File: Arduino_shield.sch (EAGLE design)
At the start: 21 parts

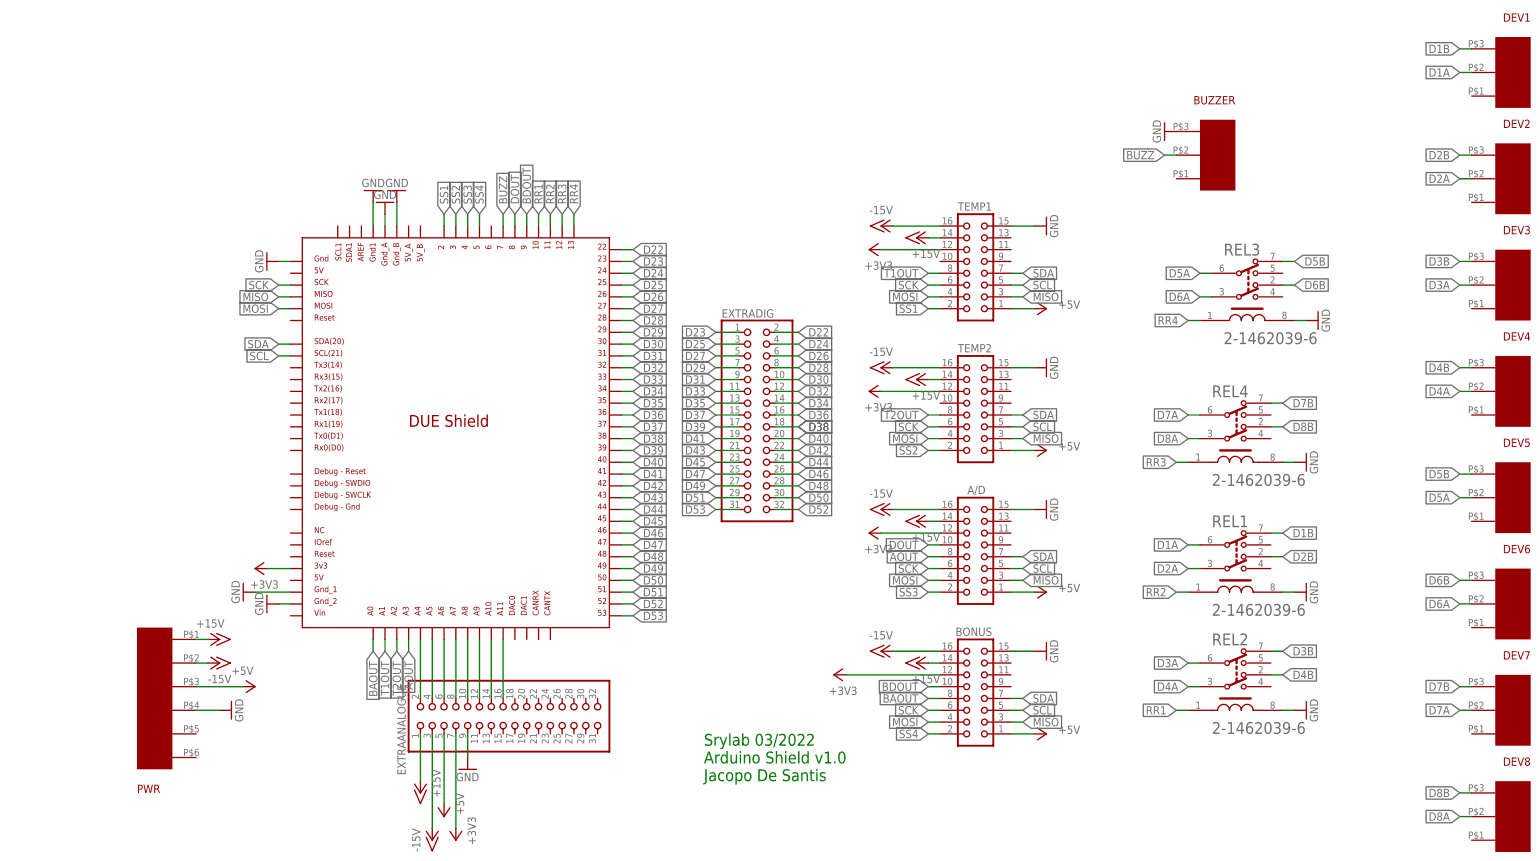
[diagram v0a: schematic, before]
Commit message: production
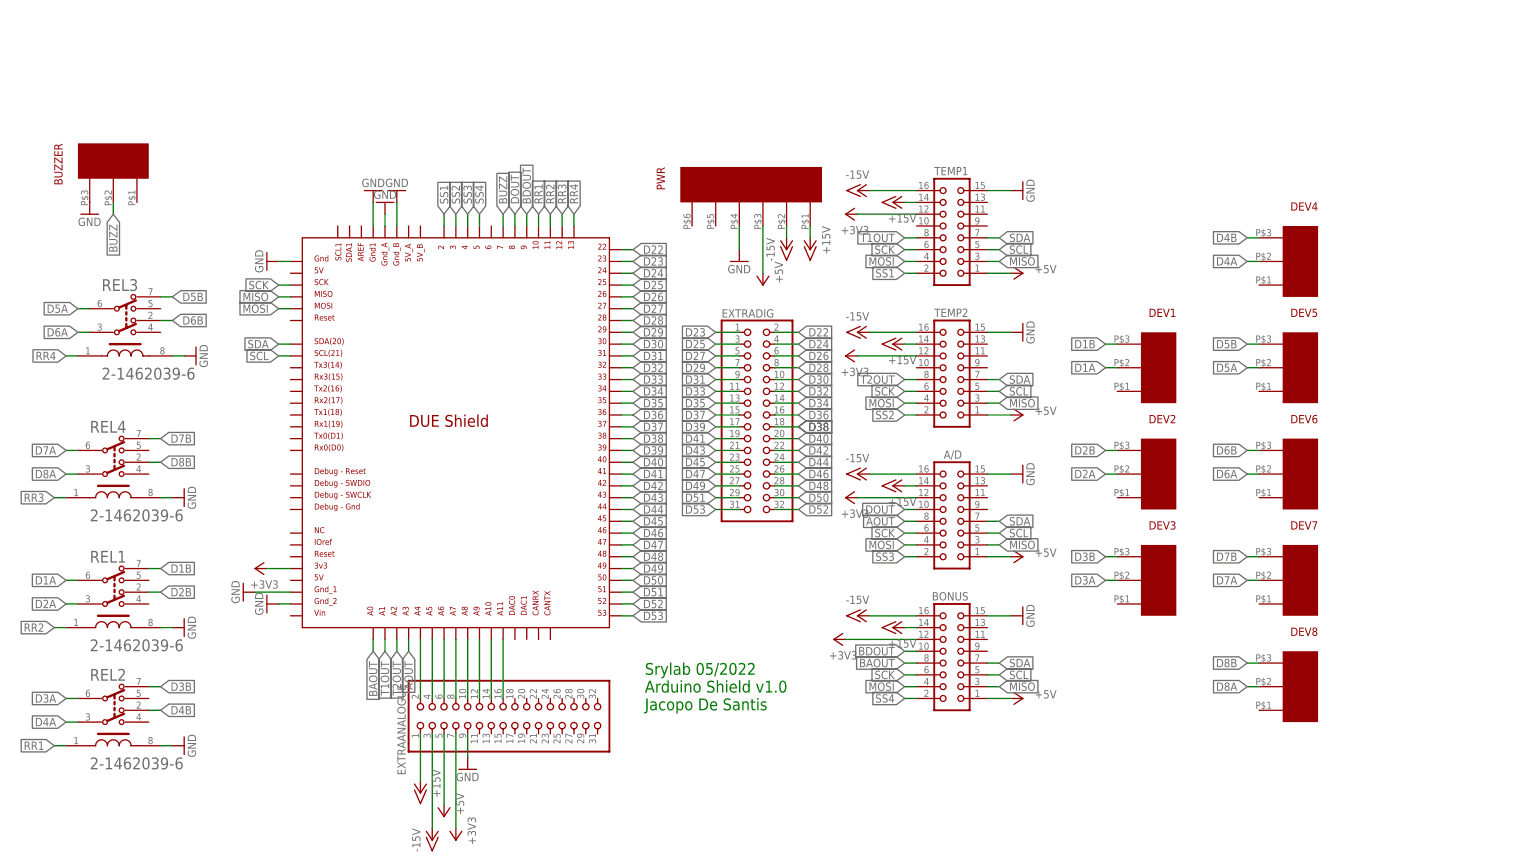
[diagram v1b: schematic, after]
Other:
- note added: "Srylab 05/2022 Arduino Shield v1.0 Jacopo De Santis"
- note removed: "Srylab 03/2022 Arduino Shield v1.0 Jacopo De Santis"
- moved on the sheet: A/D, BONUS, BUZZER, DEV1, DEV2, DEV3, DEV4, DEV5, DEV6, DEV7, DEV8, PWR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
